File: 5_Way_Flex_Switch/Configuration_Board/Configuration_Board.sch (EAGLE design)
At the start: 1 part

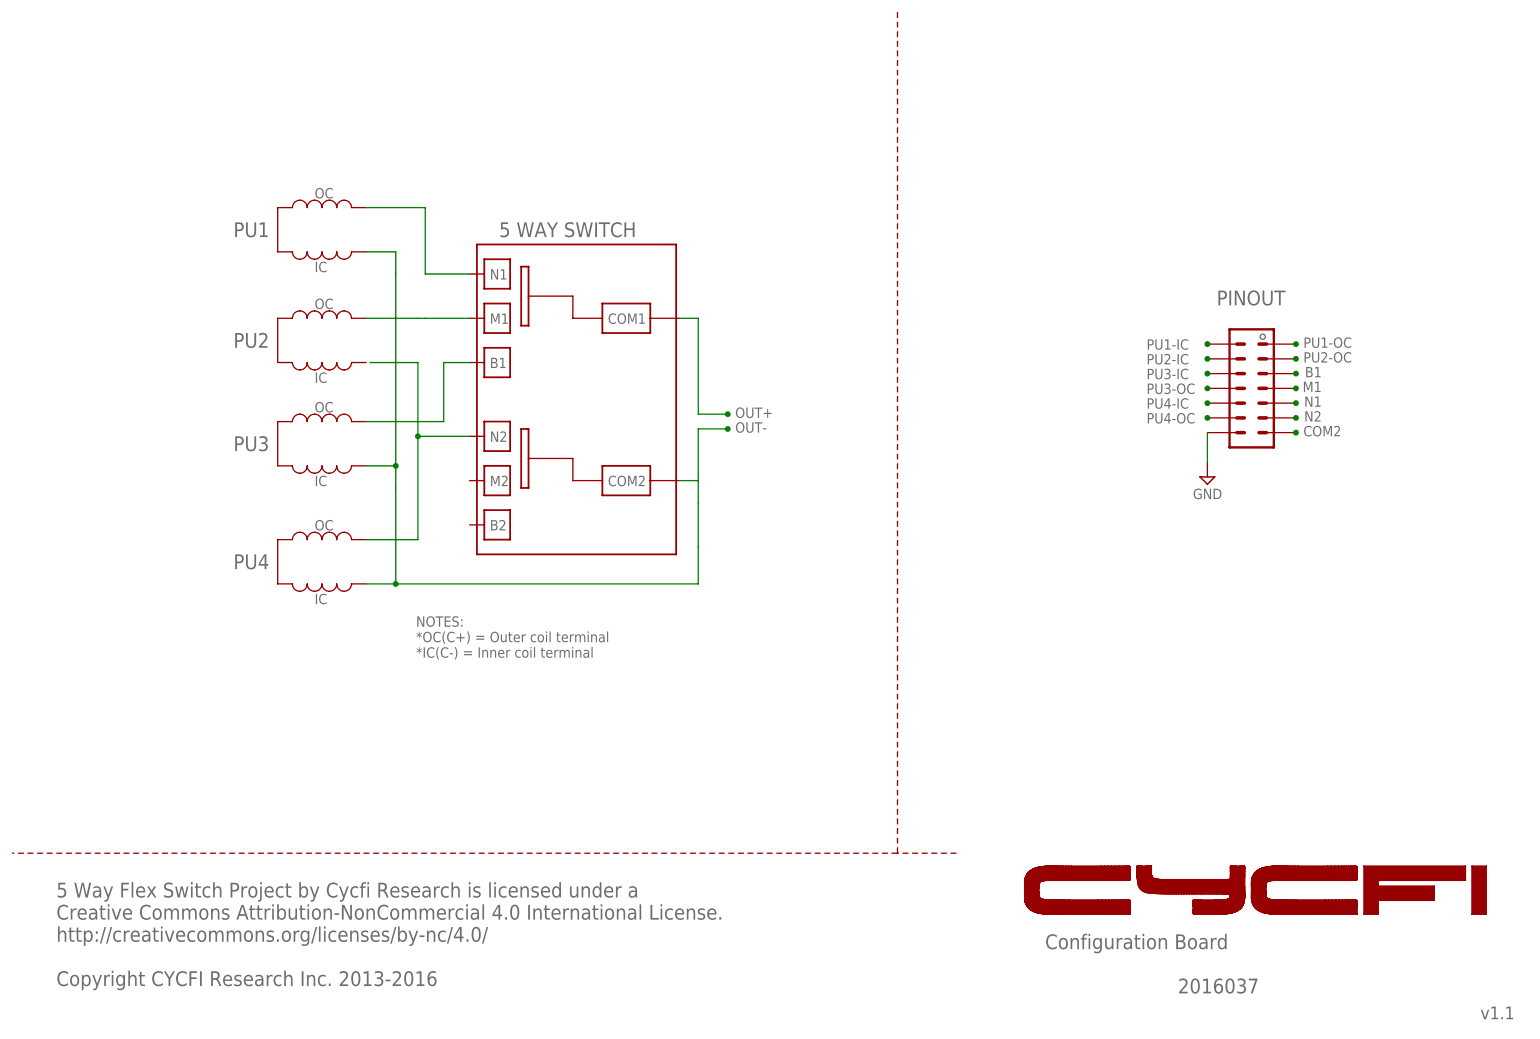
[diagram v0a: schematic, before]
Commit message: Licenses
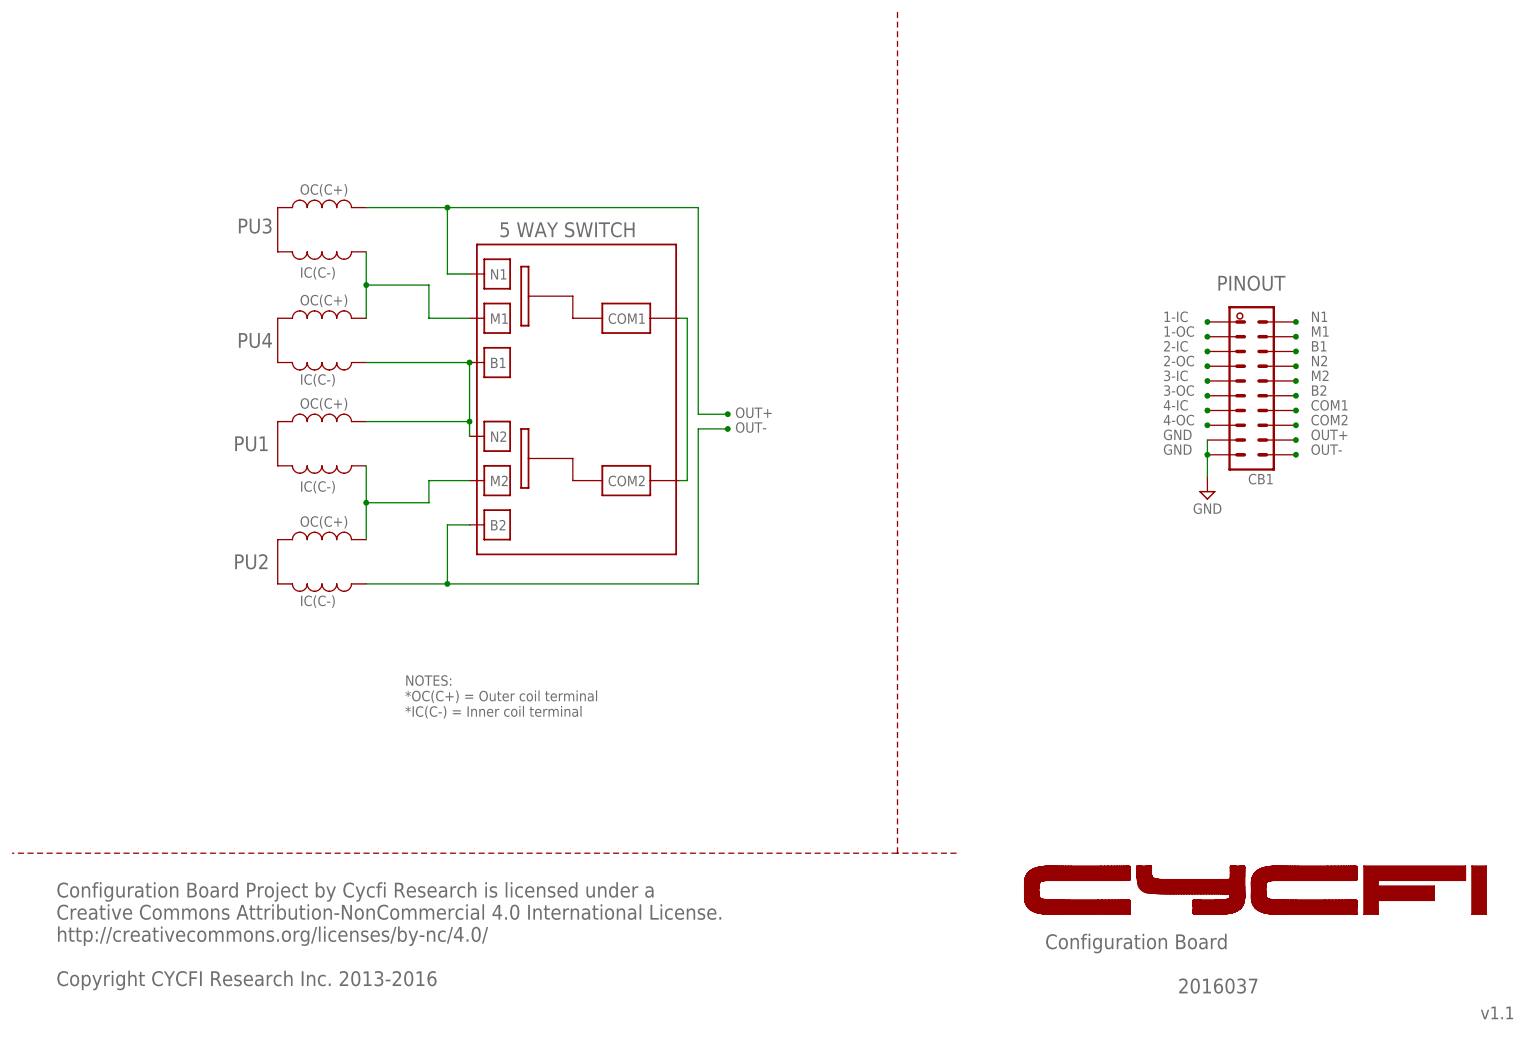
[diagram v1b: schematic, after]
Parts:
- removed U$1: CONFIGURATION_BRD_, CYCFI_Module_castellated:CONFIGURATION_BRD_
- added CB1: CONFIGURATION_BRD_CAST, CYCFI_Module_castellated:CONFIGURATION_BRD_CAST
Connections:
- removed net B1: U$1.3-OC, U$1.B
- removed net IN-: U$1.1-IC, U$1.3-IC, U$1.4-IC, U$1.IN-
- removed net M1: U$1.2-OC, U$1.M
- removed net N1: U$1.1-OC, U$1.N
- removed net N2: U$1.2-IC, U$1.4-OC, U$1.N2
- new net 1: CB1.3-OC, CB1.N1, CB1.OUT+
- new net 2: CB1.3-IC, CB1.4-OC, CB1.M1
- new net 3: CB1.1-OC, CB1.4-IC, CB1.B1, CB1.N2
- new net 4: CB1.COM1, CB1.COM2
- new net 5: CB1.1-IC, CB1.2-OC, CB1.M2
- new net 6: CB1.2-IC, CB1.B2, CB1.OUT-
- net GND: now also CB1.GND, CB1.GND1; no longer U$1.GND
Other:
- note added: "1-IC"
- note added: "1-OC"
- note added: "2-IC"
- note added: "2-OC"
- note added: "3-IC"
- note added: "3-OC"
- note added: "4-IC"
- note added: "4-OC"
- note added: "Configuration Board Project by Cycfi Research is licensed under a Creative Commons Attribution-NonCommercial 4.0 International License. http://creativecommons.org/licenses/by-nc/4.0/ Copyright CYCFI Research Inc. 2013-2016"
- note added: "GND"
- note added: "IC(C-)"
- note added: "OC(C+)"
- note removed: "5 Way Flex Switch Project by Cycfi Research is licensed under a Creative Commons Attribution-NonCommercial 4.0 International License. http://creativecommons.org/licenses/by-nc/4.0/ Copyright CYCFI Research Inc. 2013-2016"
- note removed: "IC"
- note removed: "OC"
- note removed: "PU1-IC"
- note removed: "PU1-OC"
- note removed: "PU2-IC"
- note removed: "PU2-OC"
- note removed: "PU3-IC"
- note removed: "PU3-OC"
- note removed: "PU4-IC"
- note removed: "PU4-OC"
